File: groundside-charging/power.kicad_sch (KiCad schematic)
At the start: 30 parts, among them J2 Charge Current Out (to Rocket), J3 Charge Voltage Sensing, J4 12V In, Q1 BSS138PW,115, Q2 SI4143DY-T1-GE3, Q3 SI4840BDY-T1-GE3, U1 LM317DCYR, U2 LM3478MA

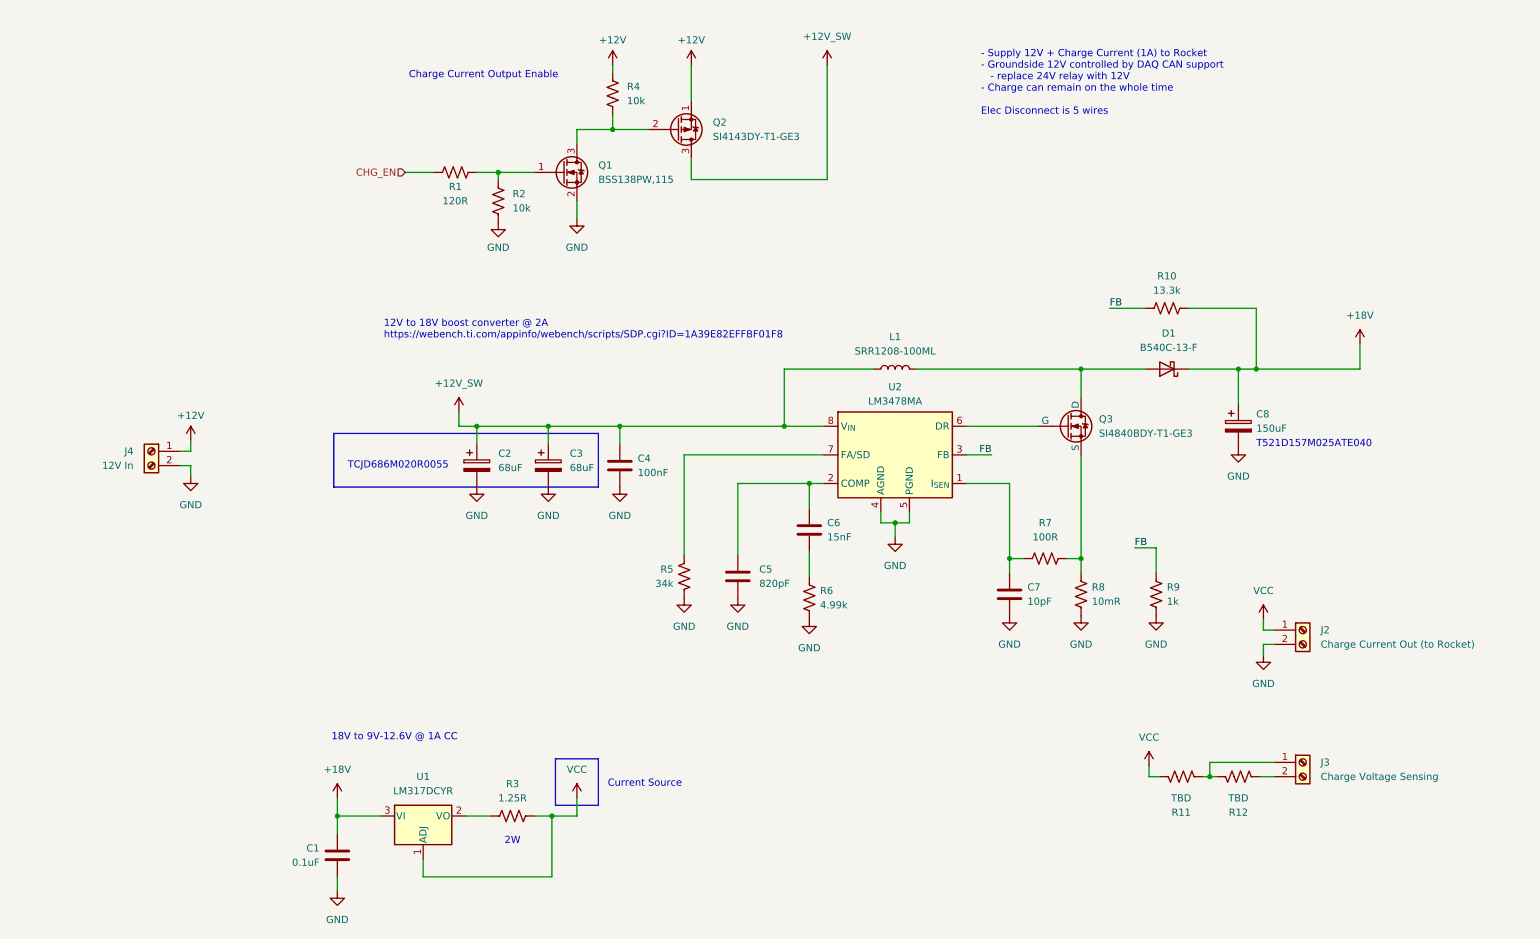
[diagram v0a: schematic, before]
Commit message: more changes
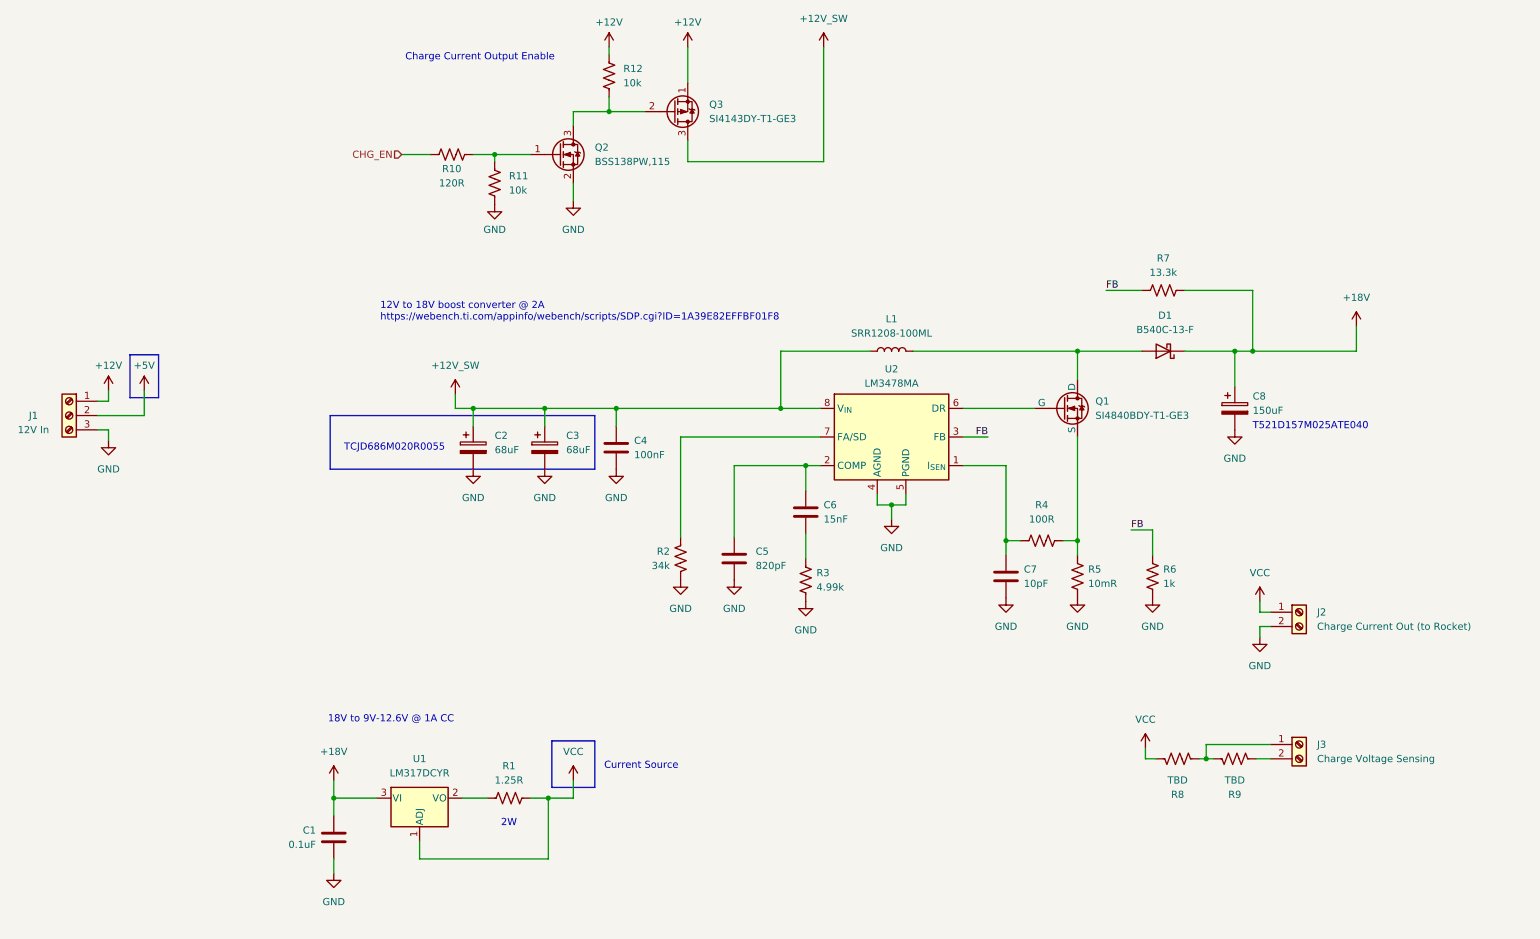
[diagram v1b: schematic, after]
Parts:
- removed J4: 12V In, TerminalBlock_Phoenix:TerminalBlock_Phoenix_PT-1,5-2-5.0-H_1x02_P5.00mm_Horizontal, symbol Connector:Screw_Terminal_01x02
- removed Q1: BSS138PW,115, Package_TO_SOT_SMD:SOT-323_SC-70_Handsoldering, symbol Device:Q_NMOS_GSD
- removed Q2: SI4143DY-T1-GE3, groundside-charging:SOIC_3DY-T1-GE3_VIS, symbol Device:Q_PMOS_SGD
- removed Q3: SI4840BDY-T1-GE3, groundside-charging:SO-8-SINGLE_MS-012_VIS, symbol Simulation_SPICE:NMOS
- added J1: 12V In, TerminalBlock_Phoenix:TerminalBlock_Phoenix_PT-1,5-3-5.0-H_1x03_P5.00mm_Horizontal, symbol Connector:Screw_Terminal_01x03
- added Q1: SI4840BDY-T1-GE3, groundside-charging:SO-8-SINGLE_MS-012_VIS, symbol Simulation_SPICE:NMOS
- added Q2: BSS138PW,115, Package_TO_SOT_SMD:SOT-323_SC-70_Handsoldering, symbol Device:Q_NMOS_GSD
- added Q3: SI4143DY-T1-GE3, groundside-charging:SOIC_3DY-T1-GE3_VIS, symbol Device:Q_PMOS_SGD
- R1: value 120R -> 1.25R; footprint Resistor_SMD:R_0805_2012Metric_Pad1.20x1.40mm_HandSolder -> Resistor_SMD:R_2512_6332Metric_Pad1.40x3.35mm_HandSolder
- R10: value 13.3k -> 120R
- R11, R12: value TBD -> 10k; footprint (none) -> Resistor_SMD:R_0805_2012Metric_Pad1.20x1.40mm_HandSolder
- R2: value 10k -> 34k
- R3: value 1.25R -> 4.99k; footprint Resistor_SMD:R_2512_6332Metric_Pad1.40x3.35mm_HandSolder -> Resistor_SMD:R_0805_2012Metric_Pad1.20x1.40mm_HandSolder
- R4: value 10k -> 100R
- R5: value 34k -> 10mR
- R6: value 4.99k -> 1k
- R7: value 100R -> 13.3k
- R8: value 10mR -> TBD; footprint Resistor_SMD:R_0805_2012Metric_Pad1.20x1.40mm_HandSolder -> (none)
- R9: value 1k -> TBD; footprint Resistor_SMD:R_0805_2012Metric_Pad1.20x1.40mm_HandSolder -> (none)
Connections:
- net +12V: now also R12.1, J1.1 (Pin_1), Q3.1 (S); no longer R4.1
- net +12V_SW: now also Q3.3 (D)
- net +18V: now also R7.2; no longer R10.2
- net CHG_EN: now also R10.1; no longer R1.1
- net FB: now also R6.1, R7.1; no longer R10.1, R9.1
- net GND: now also R11.2, R3.2, R5.1, J1.3 (Pin_3), Q2.2 (S); no longer R5.2, R8.1, R9.2
- net VCC: now also R1.2, R8.1; no longer R11.1, R3.2
- net at C6.2: now also R3.1; no longer R6.1
- net at D1.2 (A), L1.2: now also Q1.1 (D)
- net at R12.2: now also Q2.3 (D), Q3.2 (G); no longer J3.2 (Pin_2)
- net at R2.1: now also U2.7 (FA/SD); no longer R1.2
- net at R4.2: now also R5.2, Q1.3 (S)
- net at U2.6 (DR): now also Q1.2 (G)
- net at R8.2: now also J3.1 (Pin_1), R9.1; no longer R7.2
- net at C7.1, U2.1 (I_{SEN}): now also R4.1; no longer R7.1
- net at U1.2 (VO): now also R1.1; no longer R3.1
- new net: Q2.1 (G), R10.2, R11.1
- new net: J3.2 (Pin_2), R9.2
- new net +5V: J1.2 (Pin_2)
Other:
- note removed: "- Supply 12V + Charge Current (1A) to Rocket - Groundside 12V controlled by DAQ CAN support - replace 24V relay with 12V - Charge can remain on the whole time Elec Disconnect is 5 wires"
